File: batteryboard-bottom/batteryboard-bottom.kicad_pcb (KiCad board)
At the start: 2 copper layers, 45.6 x 45.6 mm, 28 parts, among them J1 SFC-110-T2-X-D-A, J2 FTS-107-01-X-DV-A, Q1 NX3008NBKS, Q2 MBT2222ADW1T1, Q3 NX3008NBKS, Q4 MBT2222ADW1T1, U1 INA219BxD

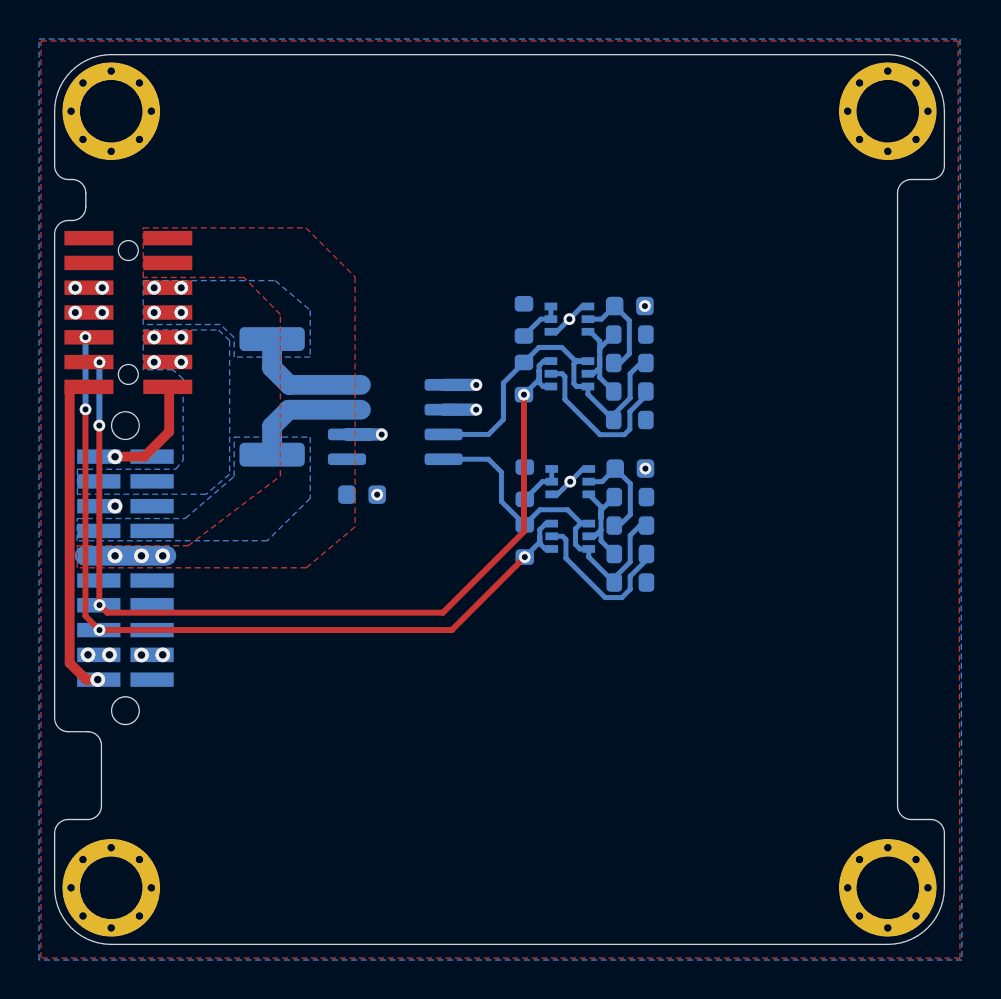
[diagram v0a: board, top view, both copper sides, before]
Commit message: Exported Gerbers
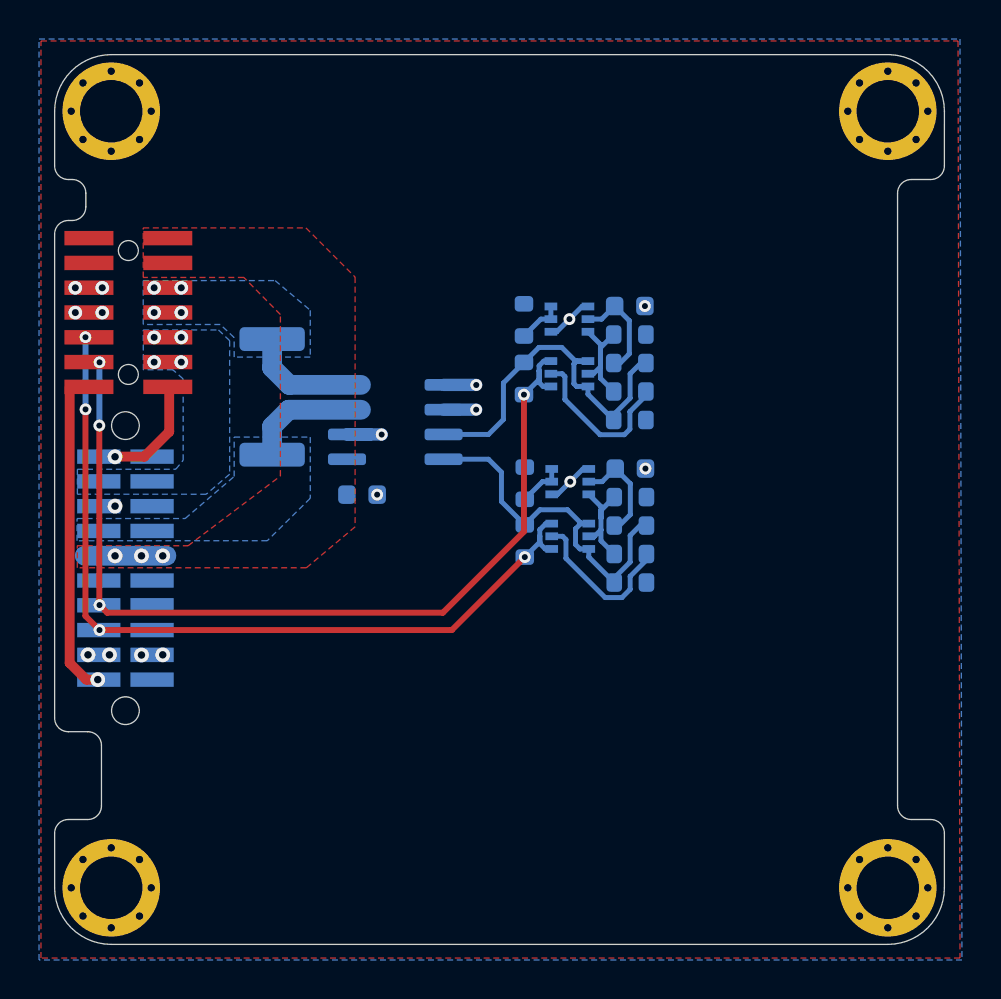
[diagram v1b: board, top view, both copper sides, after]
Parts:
- renumbered H4 to Hw
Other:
- rule pad_to_mask_clearance: 0.0508 -> 0
